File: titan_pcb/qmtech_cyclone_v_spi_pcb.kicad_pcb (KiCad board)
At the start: 2 copper layers, 146.1 x 95 mm, 44 parts, among them J1 FPGA, J10 OLED_CONN, J11 OLED_CONN, J12 CH341_PRG_CONN, J13 SPI_HEADER, J14 SPI_HEADER, J15 I2C_PULLUP, J16 I2C_PULLUP, J17 I2C_PULLUP, J18 I2C_PULLUP, J19 Barrel_Jack_MountingPin, J2 FPGA, J20 PWR_SW, J21 PWR_SW, J22 PWR_SW, J23 PWR_SW, J3 TEENSY, J4 TEENSY, J5 ESP, J6 ESP, J7 PICO, J8 PICO, J9 OLED_JMP, U1 LM1084-3.3

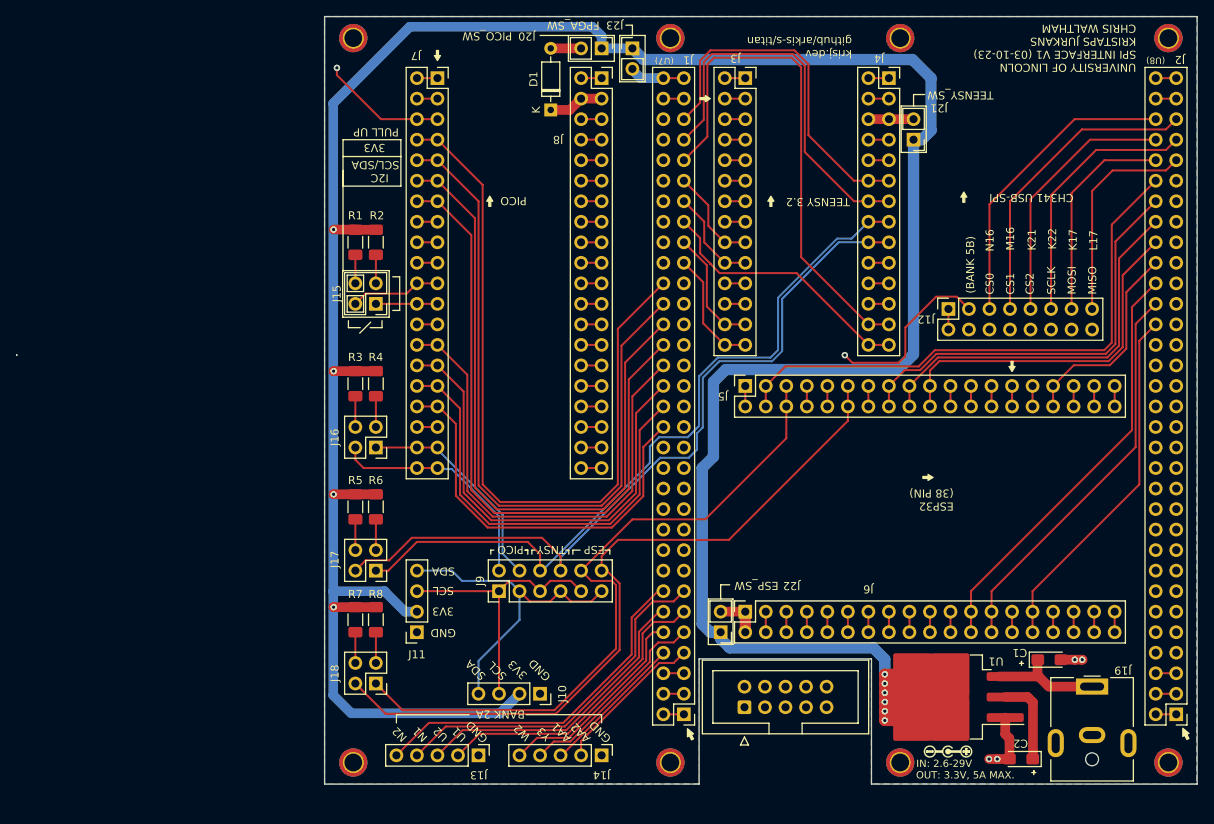
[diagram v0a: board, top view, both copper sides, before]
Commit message: updated pcb
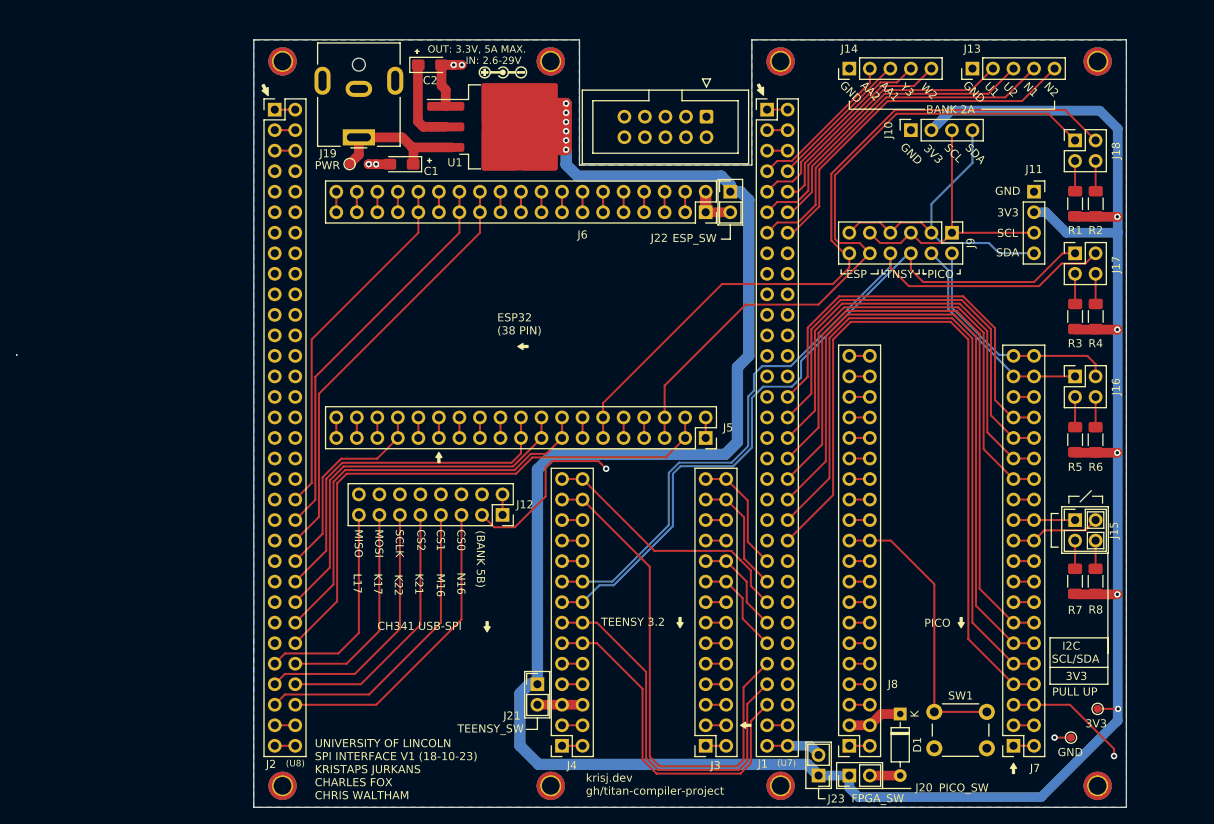
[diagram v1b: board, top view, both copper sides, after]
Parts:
- added REF**: TestPoint_Pad_D1.0mm, TestPoint:TestPoint_Pad_D1.0mm, F.Cu at (140.1, 116.2)
- added REF**: TestPoint_Pad_D1.0mm, TestPoint:TestPoint_Pad_D1.0mm, F.Cu at (136.8, 119.7)
- added REF**: TestPoint_Pad_D1.0mm, TestPoint:TestPoint_Pad_D1.0mm, F.Cu at (47.6, 48.7)
- added SW1: PICO_RESET_SW, Button_Switch_THT:SW_PUSH_6mm_H5mm, F.Cu at (119.9, 116.5)
- moved H5 143.5 mm to (39.2, 125.7), turned to 180 degrees
- moved H6 139.8 mm to (39.2, 36.0), turned to 180 degrees
- moved J2 134.4 mm to (38.3, 42.0), turned to 0 degrees
- moved H1 130.6 mm to (140.1, 125.7), turned to 180 degrees
- moved H2 126.6 mm to (140.1, 36.0), turned to 180 degrees
- moved J19 113.4 mm to (48.7, 45.4), turned to 180 degrees
- moved C2 112.9 mm to (57.5, 36.5), turned to 0 degrees
- moved J18 109.6 mm to (137.3, 45.8), turned to 0 degrees
- moved J7 109.1 mm to (129.7, 120.7), turned to 180 degrees
- moved J13 104.7 mm to (124.6, 36.9), turned to 90 degrees
- moved H7 102.2 mm to (72.4, 125.7), turned to 180 degrees
- moved C1 100.9 mm to (54.0, 48.8), turned to 180 degrees
- moved H8 97.0 mm to (72.4, 36.0), turned to 180 degrees
- moved J20 95.1 mm to (109.4, 124.4), turned to 90 degrees
- moved J17 95.0 mm to (137.3, 59.8), turned to 0 degrees
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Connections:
- R1 pad 1: Net-(J15-Pin_4) -> Net-(J18-Pin_3)
- R2 pad 1: Net-(J15-Pin_3) -> Net-(J18-Pin_4)
- R3 pad 1: Net-(J16-Pin_4) -> Net-(J17-Pin_3)
- R4 pad 1: Net-(J16-Pin_3) -> Net-(J17-Pin_4)
- R5 pad 1: Net-(J17-Pin_4) -> Net-(J16-Pin_3)
- R6 pad 1: Net-(J17-Pin_3) -> Net-(J16-Pin_4)
- R7 pad 1: Net-(J18-Pin_4) -> Net-(J15-Pin_3)
- R8 pad 1: Net-(J18-Pin_3) -> Net-(J15-Pin_4)
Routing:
- net PICO_RUN: track 2.54 -> 35.1 mm
- net Net-(U1-VI): track 14.5 -> 17.8 mm
- net 3V3: track 370.4 -> 372.9 mm, vias 10 -> 11
- net GND: track 91.2 -> 93.2 mm, vias 6 -> 7
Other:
- board size 146.1 x 95 mm -> 137.4 x 95 mm
- board text added: "PWR"
- board text added: "UNIVERSITY OF LINCOLN SPI INTERFACE V1 (18-10-23) KRISTAPS JURKANS CHARLES FOX CHRIS WALTHAM"
- board text added: "krisj.dev gh/titan-compiler-project"
- board text removed: "UNIVERSITY OF LINCOLN SPI INTERFACE V1 (03-10-23) KRISTAPS JURKANS CHRIS WALTHAM"
- board text removed: "krisj.dev github/arkis-s/titan"
